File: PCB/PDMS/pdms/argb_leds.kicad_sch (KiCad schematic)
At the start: 19 parts

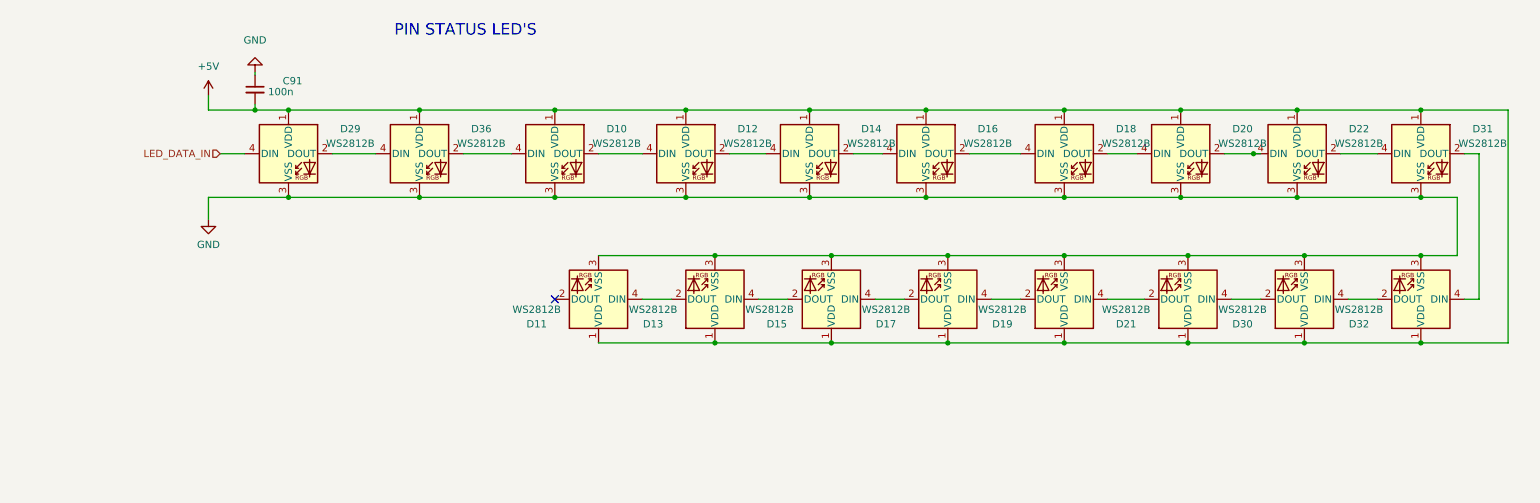
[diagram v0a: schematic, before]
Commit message: Major changes with new switch
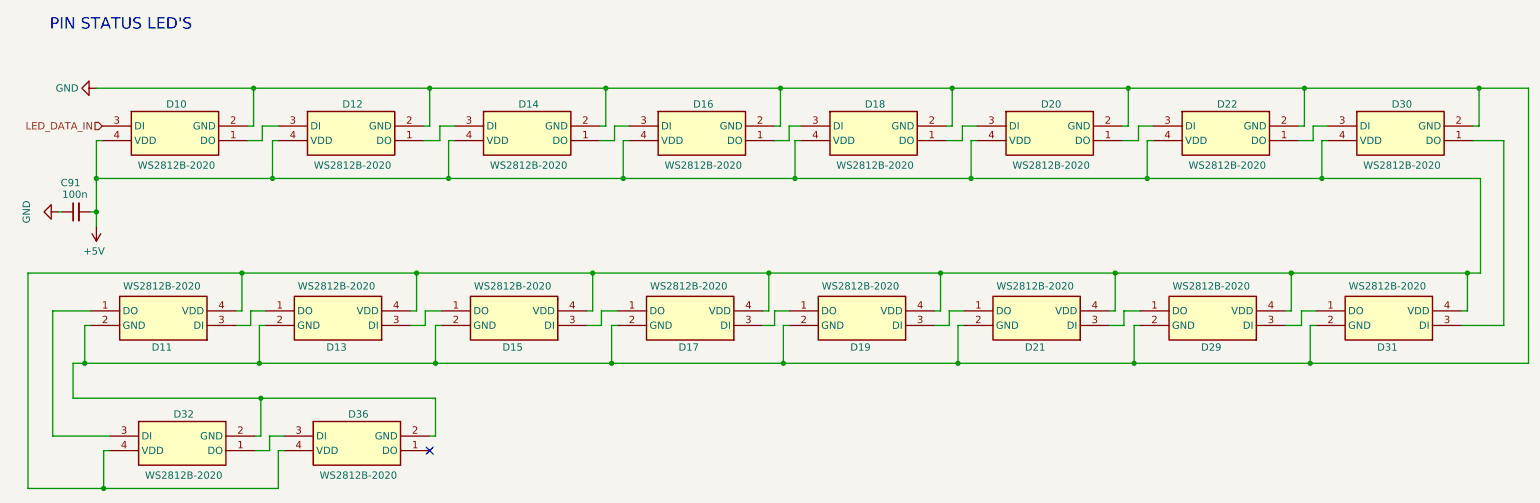
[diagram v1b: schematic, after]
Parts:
- removed D10, D11, D12, D13, D14, D15, D16, D17, D18, D19, D20, D21, D22, D29, D30, D31, D32, D36: WS2812B, LED_SMD:LED_WS2812B-2020_PLCC4_2.0x2.0mm, symbol LED:WS2812B
- added D10, D11, D12, D13, D14, D15, D16, D17, D18, D19, D20, D21, D22, D29, D30, D31, D32, D36: WS2812B-2020, PDMS_Additional:WS2812B2020, symbol pdms_additional:WS2812B-2020
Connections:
- net +5V: now also D10.4 (VDD), D11.4 (VDD), D12.4 (VDD), D13.4 (VDD), D14.4 (VDD), D15.4 (VDD), D16.4 (VDD), D17.4 (VDD), D18.4 (VDD), D19.4 (VDD), D20.4 (VDD), D21.4 (VDD), D22.4 (VDD), D29.4 (VDD), D30.4 (VDD), D31.4 (VDD), D32.4 (VDD), D36.4 (VDD)
- net GND: now also D10.2 (GND), D11.2 (GND), D12.2 (GND), D13.2 (GND), D14.2 (GND), D15.2 (GND), D16.2 (GND), D17.2 (GND), D18.2 (GND), D19.2 (GND), D20.2 (GND), D21.2 (GND), D22.2 (GND), D29.2 (GND), D30.2 (GND), D31.2 (GND), D32.2 (GND), D36.2 (GND)
- net LED_DATA_IN: now also D10.3 (DI)
- new net: D29.3 (DI), D31.1 (DO)
- new net: D30.1 (DO), D31.3 (DI)
- new net: D11.1 (DO), D32.3 (DI)
- new net: D11.3 (DI), D13.1 (DO)
- new net: D22.1 (DO), D30.3 (DI)
- new net: D20.1 (DO), D22.3 (DI)
- new net: D32.1 (DO), D36.3 (DI)
- new net: D12.1 (DO), D14.3 (DI)
- new net: D10.1 (DO), D12.3 (DI)
- new net: D13.3 (DI), D15.1 (DO)
- new net: D15.3 (DI), D17.1 (DO)
- new net: D17.3 (DI), D19.1 (DO)
- new net: D19.3 (DI), D21.1 (DO)
- new net: D16.1 (DO), D18.3 (DI)
- new net: D14.1 (DO), D16.3 (DI)
- new net: D18.1 (DO), D20.3 (DI)
- new net: D21.3 (DI), D29.1 (DO)
